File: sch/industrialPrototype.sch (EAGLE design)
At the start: 13 parts, among them IC1 LD1117V33C, U1 PIC16F1825-I/SL

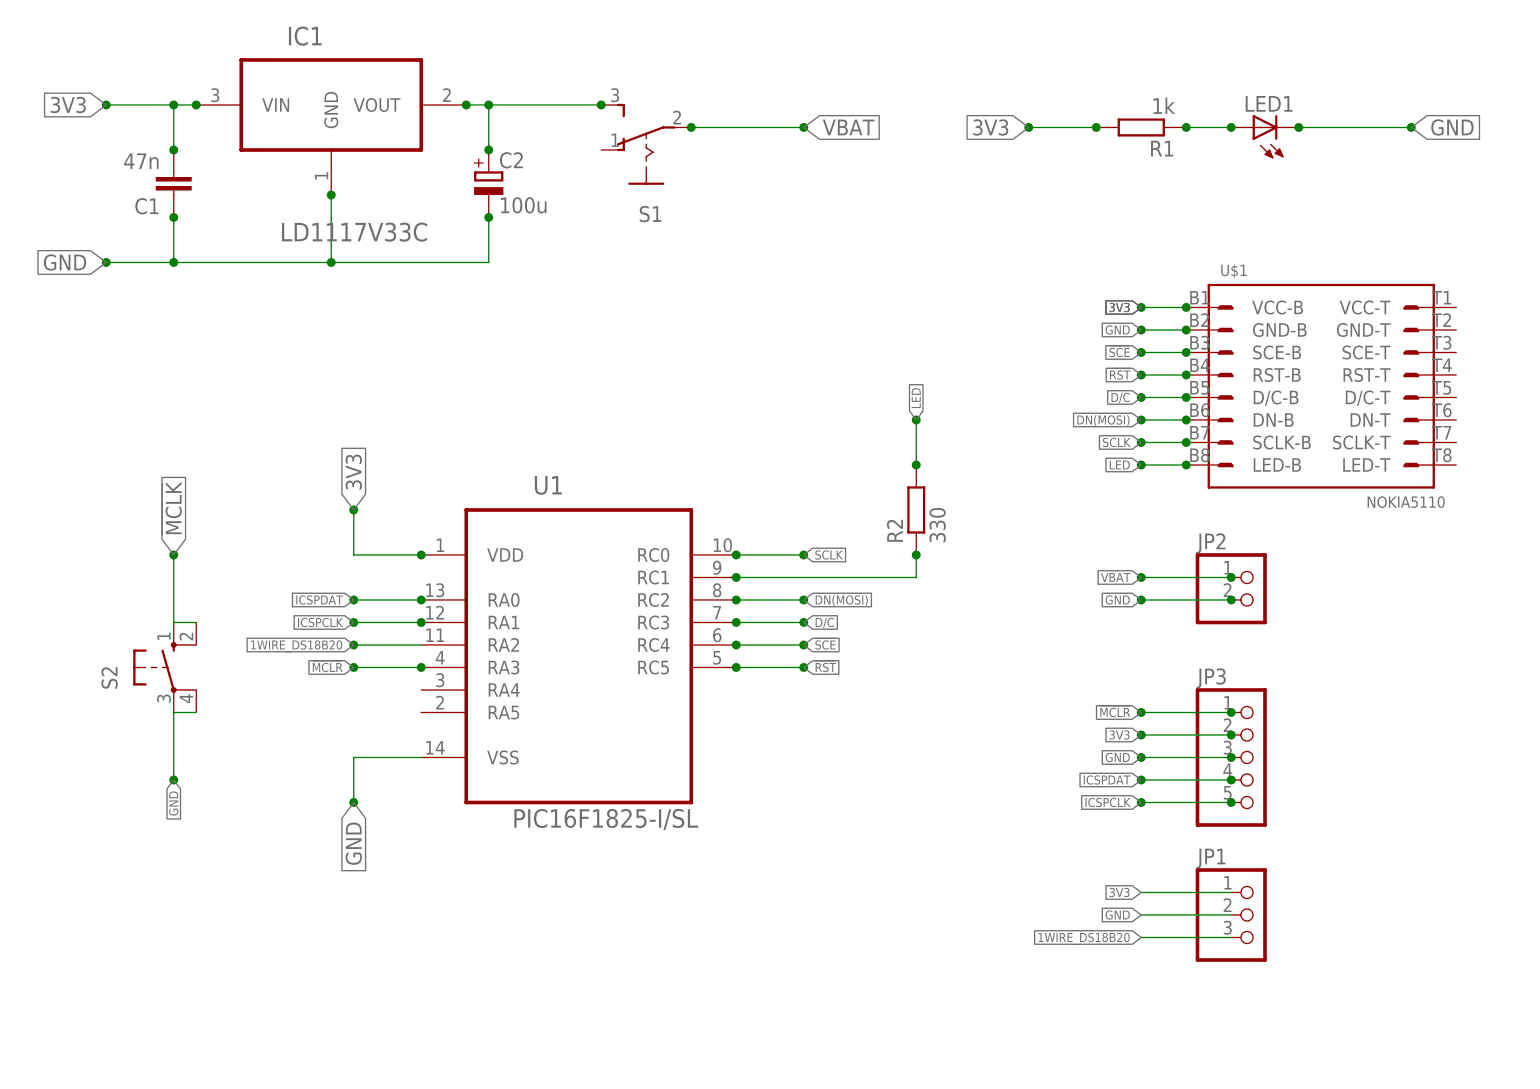
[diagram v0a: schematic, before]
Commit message: Final Version of the Schematic and Board
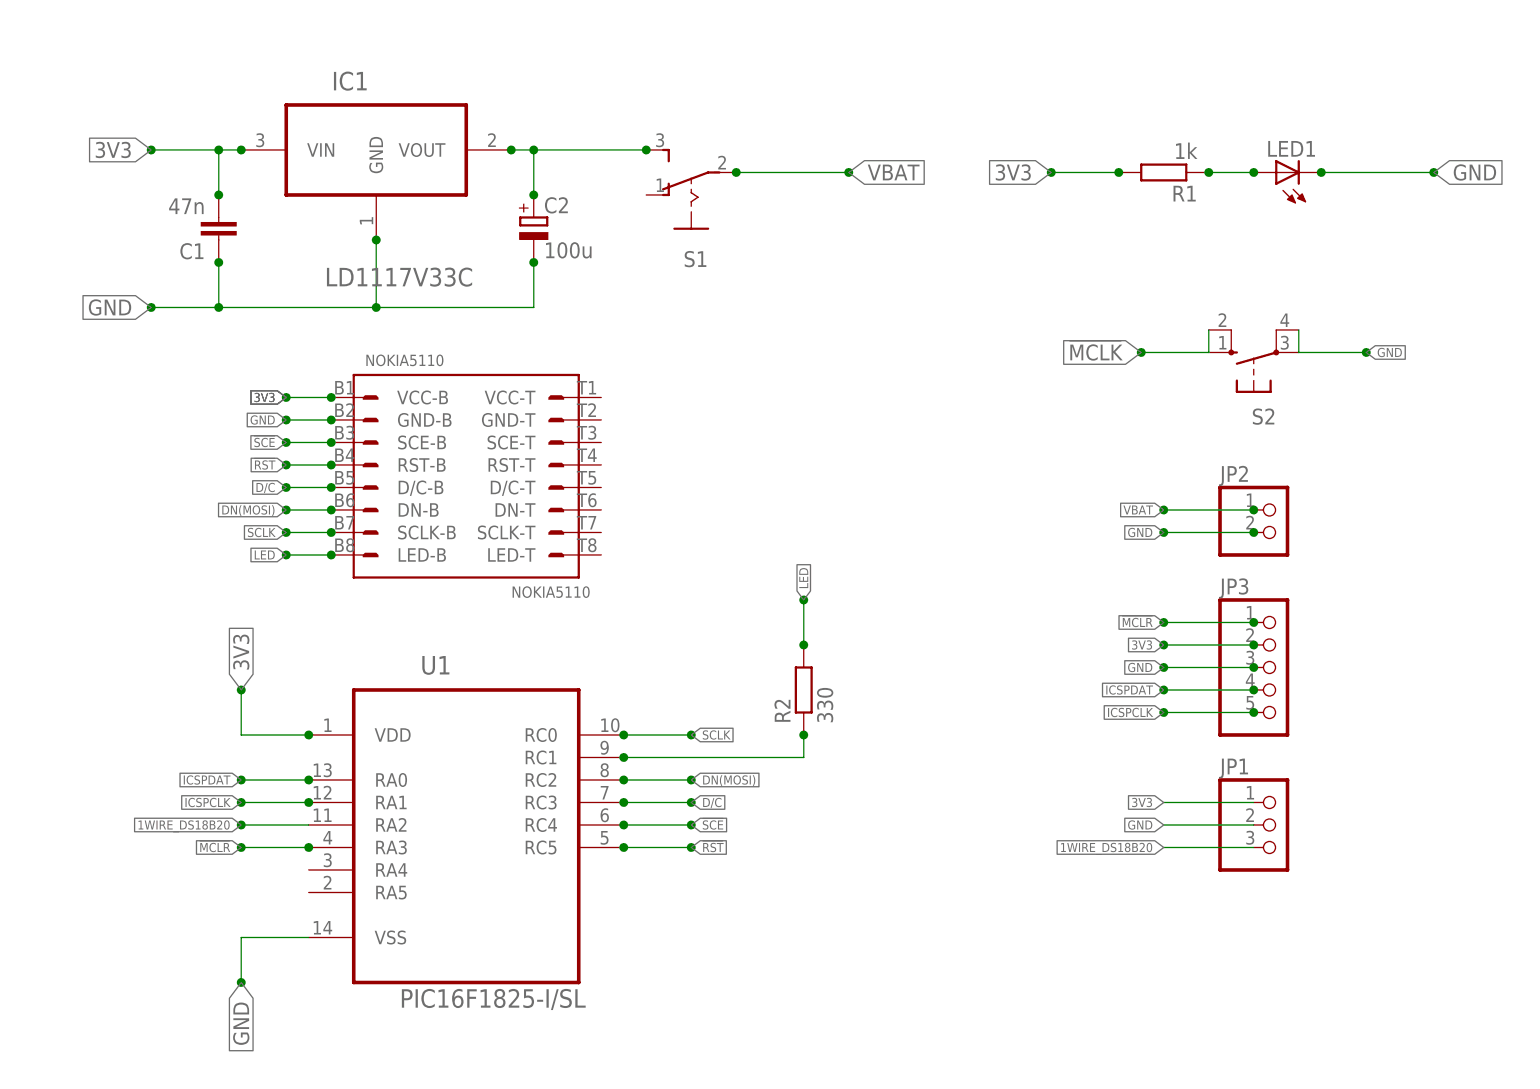
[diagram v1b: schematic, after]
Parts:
- removed U$1: NOKIA5110, CustomLib:NOKIA5110
- added NOKIA5110: NOKIA5110, CustomLib:NOKIA5110
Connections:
- net !RST!: now also NOKIA5110.RST-B; no longer U$1.RST-B
- net !SCE!: now also NOKIA5110.SCE-B; no longer U$1.SCE-B
- net 3V3: now also NOKIA5110.VCC-B; no longer U$1.VCC-B
- net D/C: now also NOKIA5110.D/C-B; no longer U$1.D/C-B
- net DN(MOSI): now also NOKIA5110.DN-B; no longer U$1.DN-B
- net GND: now also NOKIA5110.GND-B; no longer U$1.GND-B
- net LED: now also NOKIA5110.LED-B; no longer U$1.LED-B
- net SCLK: now also NOKIA5110.SCLK-B; no longer U$1.SCLK-B
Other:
- moved on the sheet: C1, C2, IC1, JP1, JP2, JP3, LED1, R1, R2, S1, S2, U1
